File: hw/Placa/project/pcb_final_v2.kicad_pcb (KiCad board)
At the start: 2 copper layers, 22 parts, among them J1 pin_socket-bluepill, J10 tcrt5000_conector_2, J11 tcrt5000_conector_3, J12 tcrt5000_conector_1, J2 pin_socket-bluepill, J9 tof-connector_3, SW2 key, U2 Receptor IR, U4 AMS1117-3.3

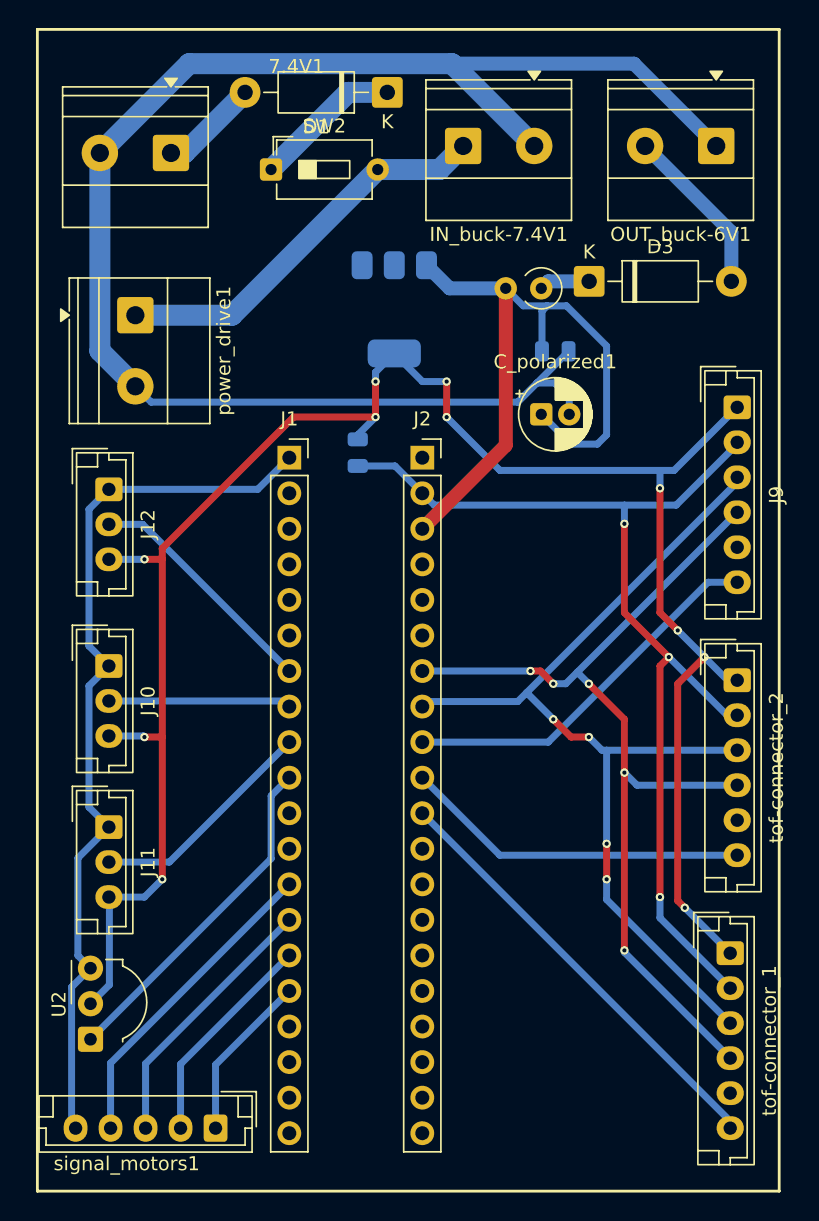
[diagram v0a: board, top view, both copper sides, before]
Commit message: atualização pcb
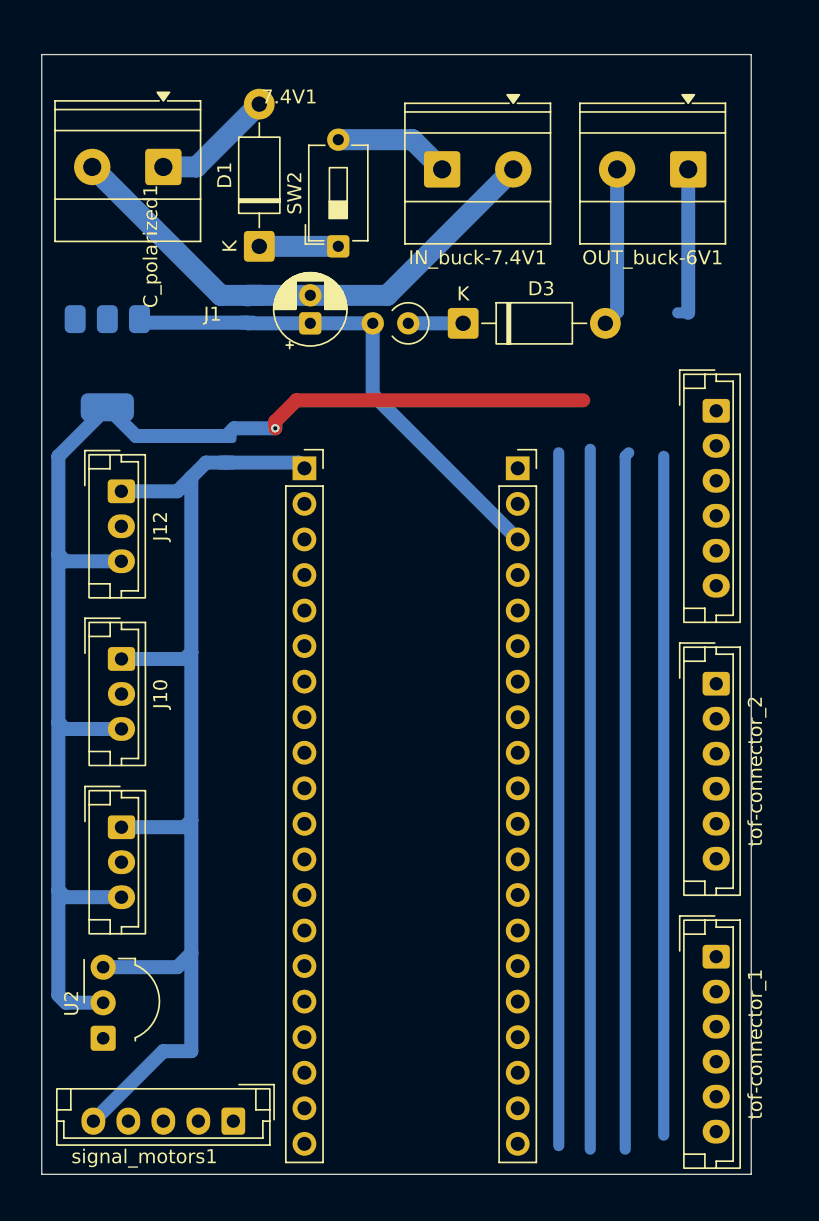
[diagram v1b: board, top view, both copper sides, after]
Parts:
- removed power_drive1: KRE borne, TerminalBlock_Phoenix:TerminalBlock_Phoenix_MKDS-1,5-2-5.08_1x02_P5.08mm_Horizontal
- moved C2 22.2 mm to (128.0, 68.5), turned to -90 degrees
- moved U4 20.9 mm to (118.0, 72.3)
- moved C_polarized1 17.7 mm to (132.5, 69.5), turned to 90 degrees
- moved D1 14.3 mm to (128.9, 64.0), turned to 90 degrees
- moved L1 9.82 mm to (139.5, 69.5)
- moved D3 9.49 mm to (143.4, 69.5)
- moved C3 9.39 mm to (126.5, 78.5)
- moved SW2 7.29 mm to (134.5, 64.0), turned to 90 degrees
- moved J2 6.86 mm to (147.3, 79.9)
- moved OUT_buck-6V1 2.61 mm to (159.5, 58.5)
- moved IN_buck-7.4V1 2.25 mm to (147.0, 58.5)
- moved J9 1.52 mm to (161.5, 75.8)
- moved tof-connector_2 1.52 mm to (161.5, 95.2)
- moved signal_motors1 1.36 mm to (127.0, 126.5)
- moved J1 1.32 mm to (132.1, 79.9)
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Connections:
- OUT_buck-6V1 pad 1: GNDPWR -> GNDS
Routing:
- net (no net): track 0.00 -> 197.9 mm
- net GNDPWR: track 112.0 -> 38.6 mm
- net I2C1_SCL: track 69.4 -> 0.00 mm, vias 4 -> 0
- net I2C1_SDA: track 68.5 -> 0.00 mm, vias 5 -> 0
- net GNDS: track 138.8 -> 92.3 mm, vias 3 -> 0
- net +3V3: track 142.7 -> 97.2 mm, vias 11 -> 1
- net XSHUT1: track 31.6 -> 0.00 mm
- net XSHUT3: track 27.2 -> 0.00 mm
- net XSHUT2: track 24.8 -> 0.00 mm
- net D4: track 24.6 -> 0.00 mm
- net MB-: track 22.7 -> 0.00 mm
- net IN-BUCK: track 28.4 -> 8.30 mm
- net MB+: track 19.1 -> 0.00 mm
- net D1: track 17.2 -> 0.00 mm
- net D3: track 16.4 -> 0.00 mm
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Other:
- board outline added: 50.7 x 80 mm
